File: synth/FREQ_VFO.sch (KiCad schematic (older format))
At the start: 37 parts

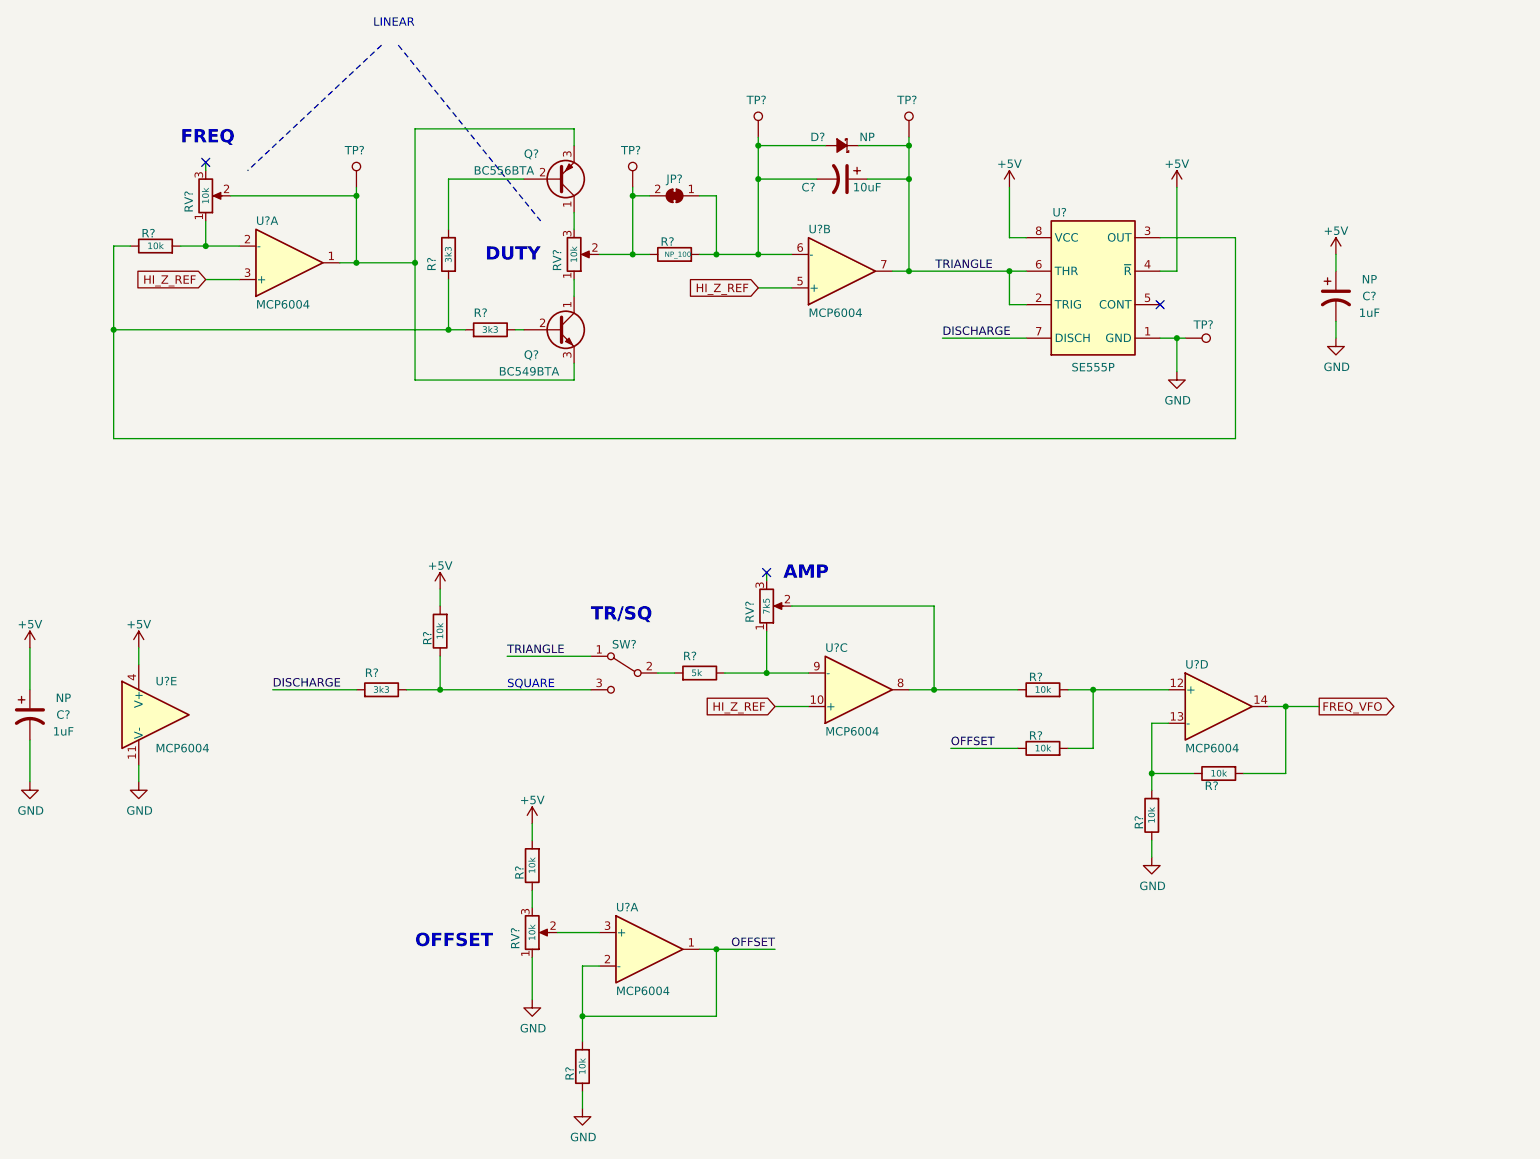
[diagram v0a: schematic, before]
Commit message: automated commit
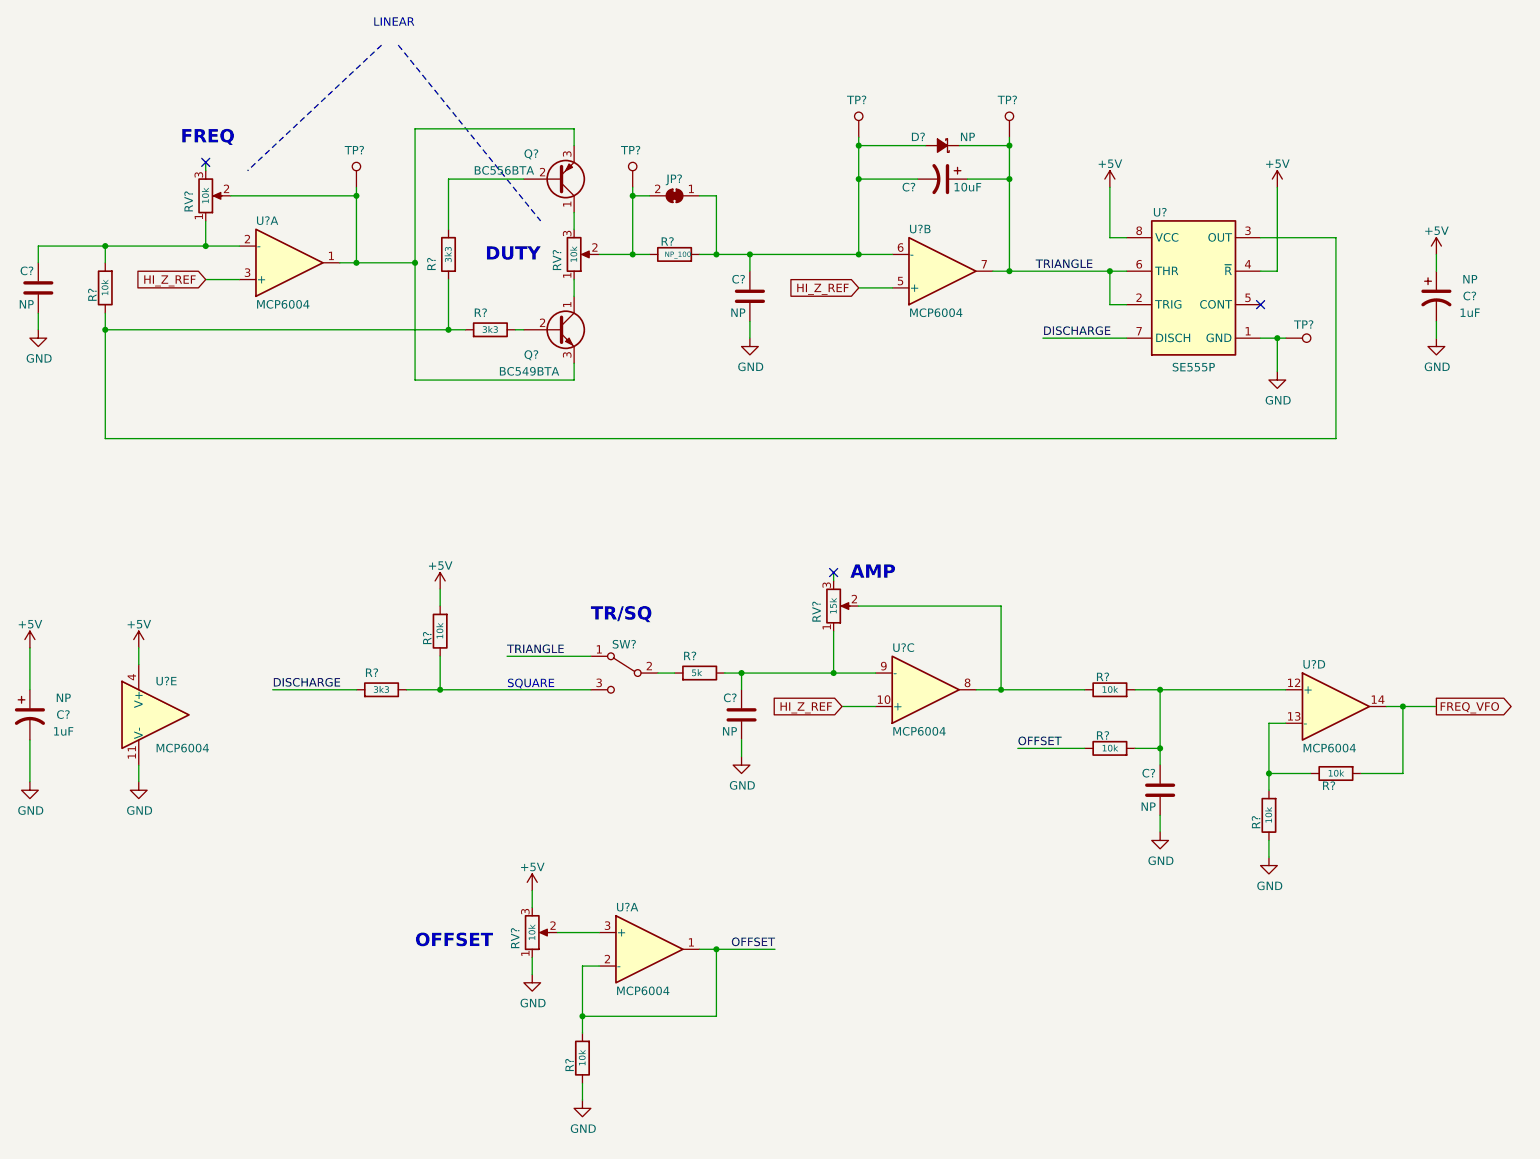
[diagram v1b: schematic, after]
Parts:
- removed R?: 10k, symbol Device:R
- added C? (x4): NP, symbol Device:C
- RV?: value 7k5 -> 15k
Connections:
- net +5V: now also RV?.3
- net GND: now also C?.2, C?.2, C?.2, C?.2
- net at C?.2, D?.2 (A), JP?.1 (A)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: now also C?.1
- net at R?.2, RV?.1, U?.2 (-): now also C?.1
- net at R?.2, R?.2, U?.12 (+): now also C?.1
- net at R?.1, RV?.1, U?.9 (-): now also C?.1
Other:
- moved on the sheet: C?, D?, R?, RV?, TP?, U?, U?B, U?C, U?D
